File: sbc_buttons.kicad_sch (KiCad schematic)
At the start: 18 parts, among them J8 FP Power Switch, SW1 SMD_4.6x2.8mm_h2.5mm

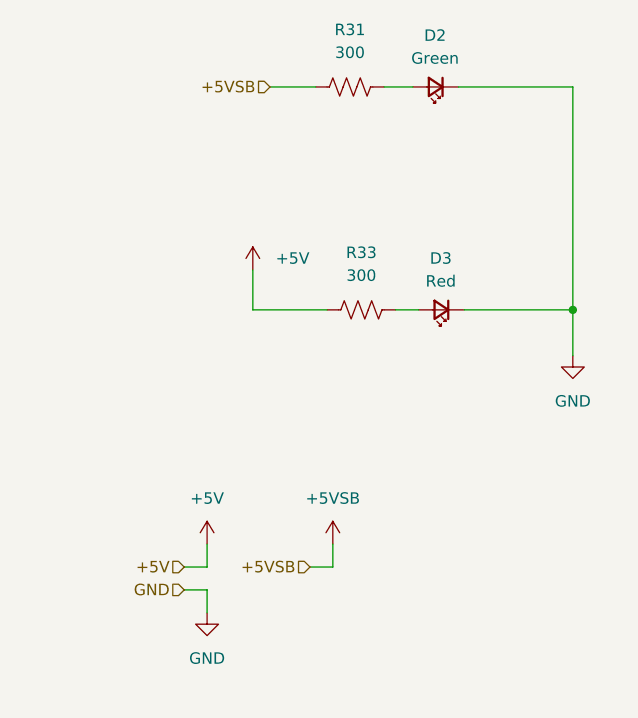
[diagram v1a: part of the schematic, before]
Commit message: rev A3 pcb, added a fun logo to the BIOS startup
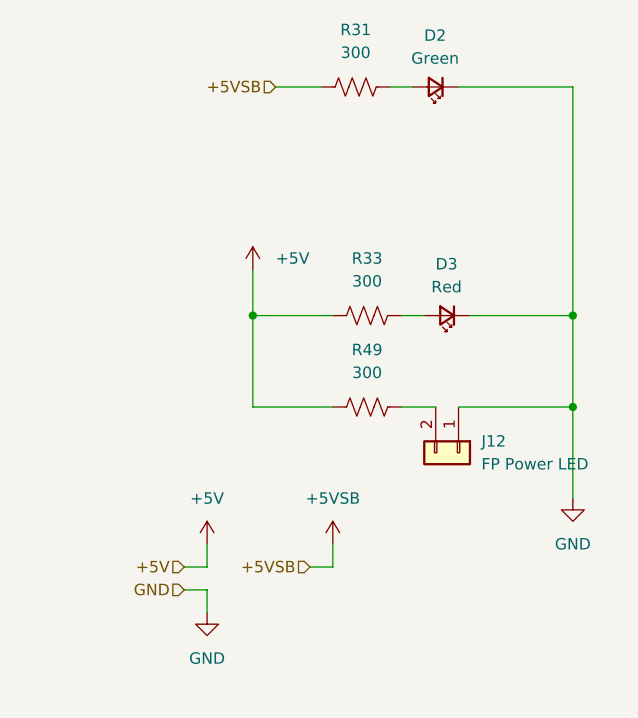
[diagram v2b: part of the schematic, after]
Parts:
- added J12: FP Power LED, Connector_PinHeader_2.54mm:PinHeader_1x02_P2.54mm_Vertical, symbol Connector_Generic:Conn_01x02
- added R49: 300, Resistor_SMD:R_0805_2012Metric, symbol Device:R_US
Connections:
- net +5V: now also R49.1
- net GND: now also J12.1 (Pin_1)
- new net: J12.2 (Pin_2), R49.2
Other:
- moved on the sheet: D3, R31, R33
